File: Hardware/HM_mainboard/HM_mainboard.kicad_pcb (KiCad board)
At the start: 2 copper layers, 80 x 55 mm, 65 parts, among them J1 JST PH2P ST90, J2 USB4105-GF-A, J3 Conn_01x04, J4 54-00174, J5 54-00174, J6 54-00174, J7 54-00174, Q1 PMOS AS3401, U1 MCP73831-2, U2 TC1262-33, U3 ESP32-S3-WROOM-1, U4 WE-TVS-824015043, U5 MC6470, U6 BNO055, Y1 32.768 kHz

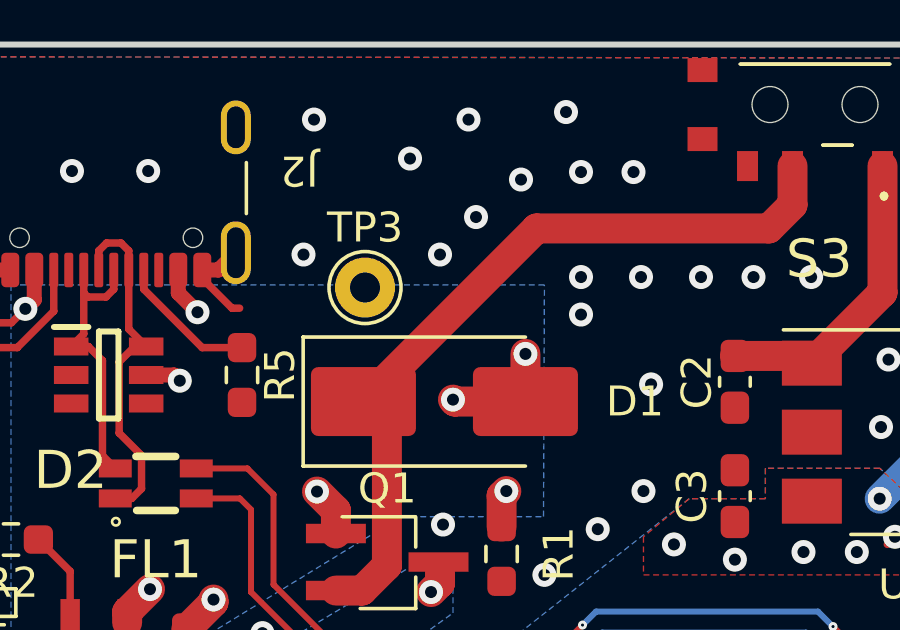
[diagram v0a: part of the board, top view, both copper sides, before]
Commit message: Added gerber files and schematic printed to pdf
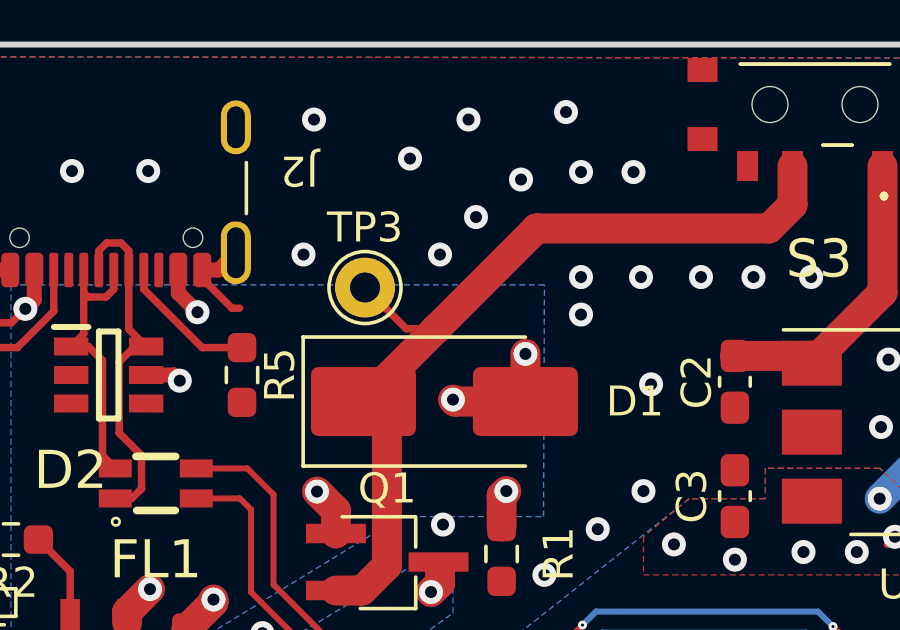
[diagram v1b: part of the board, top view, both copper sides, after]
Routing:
- net /Battery_and_Power_Managment/V_PWR_SWITCH: track 26.4 -> 29.4 mm
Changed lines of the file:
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@@
       (drillshape 0)
       (scaleselection 1)
-      (outputdirectory "")
+      (outputdirectory "Gerber/V1.0.1/")
     )
   )
@@
   (segment (start 183.03 108.745) (end 186.68 112.395) (width 0.25) (layer "F.Cu") (net 34))
   (segment (start 183.03 107.95) (end 183.03 108.745) (width 0.25) (layer "F.Cu") (net 34))
+  (segment (start 138.8 81.1) (end 140.174 82.474) (width 0.25) (layer "F.Cu") (net 35))
   (segment (start 139.53 85.682) (end 138.748 84.9) (width 1) (layer "F.Cu") (net 35))
   (segment (start 139.53 90.37) (end 139.53 85.682) (width 1) (layer "F.Cu") (net 35))
@@
   (segment (start 137.83 91.2) (end 138.7 91.2) (width 1) (layer "F.Cu") (net 35))
   (segment (start 144.518 79.13) (end 152.264 79.13) (width 1) (layer "F.Cu") (net 35))
-  (segment (start 138.748 84.9) (end 144.518 79.13) (width 1) (layer "F.Cu") (net 35))
   (segment (start 153.05 78.344) (end 153.05 77.05) (width 1) (layer "F.Cu") (net 35))
+  (segment (start 141.174 82.474) (end 144.518 79.13) (width 1) (layer "F.Cu") (net 35))
+  (segment (start 138.748 84.9) (end 141.174 82.474) (width 1) (layer "F.Cu") (net 35))
   (segment (start 138.7 91.2) (end 139.53 90.37) (width 1) (layer "F.Cu") (net 35))
+  (segment (start 140.174 82.474) (end 141.174 82.474) (width 0.25) (layer "F.Cu") (net 35))
   (segment (start 168 105.5) (end 166.5 107) (width 0.25) (layer "F.Cu") (net 36))
   (segment (start 153.35 107) (end 150.885305 109.464695) (width 0.25) (layer "F.Cu") (net 36))
